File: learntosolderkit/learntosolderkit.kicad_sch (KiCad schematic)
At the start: 11 parts, among them J1 Barrel_Jack, SW1 SW_Push, SW2 SW_Push, SW3 SW_Push, U1 NE555P

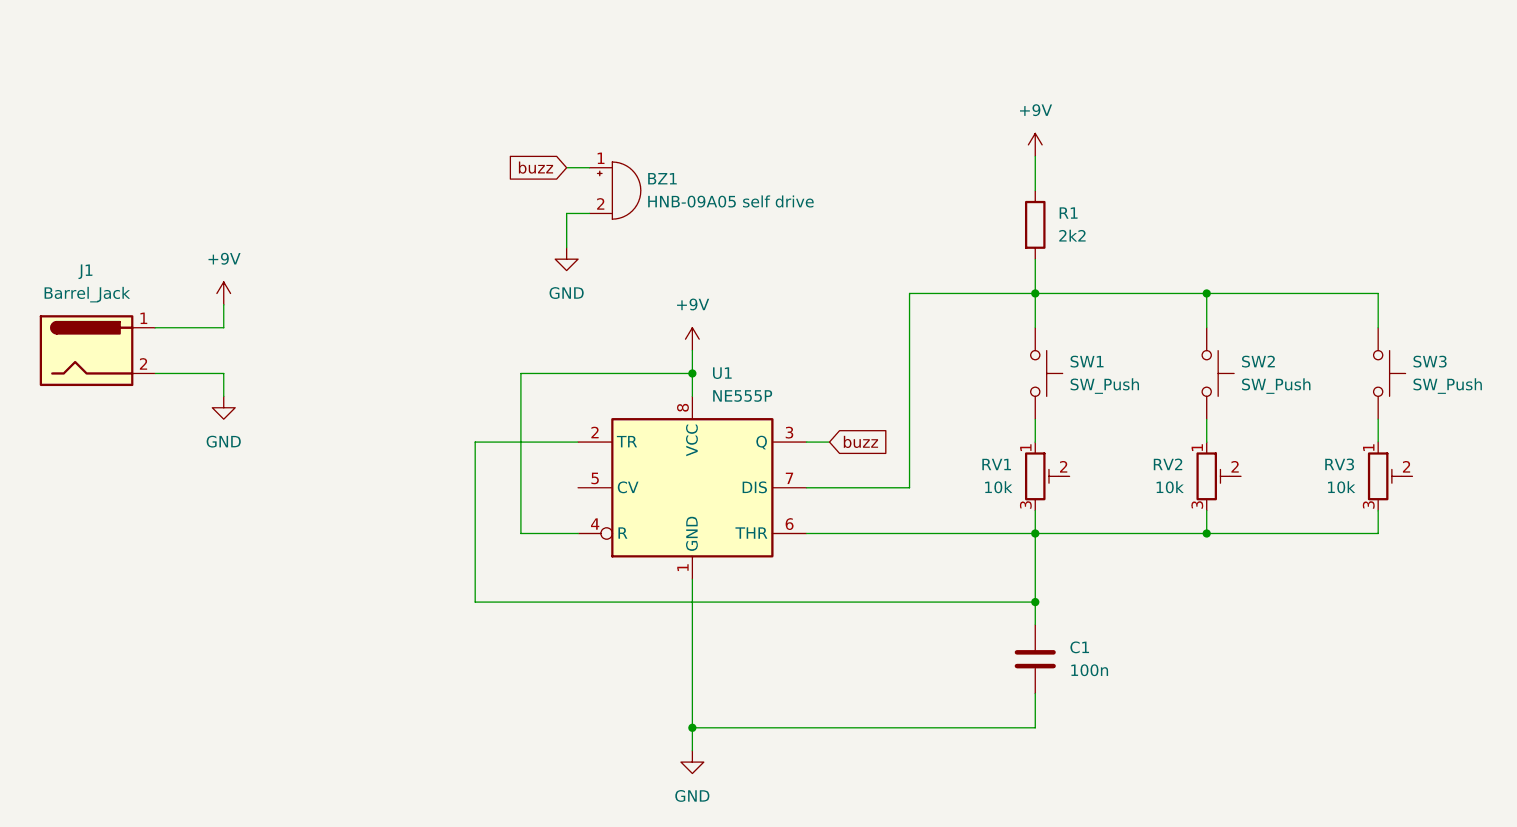
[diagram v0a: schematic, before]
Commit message: Finish up
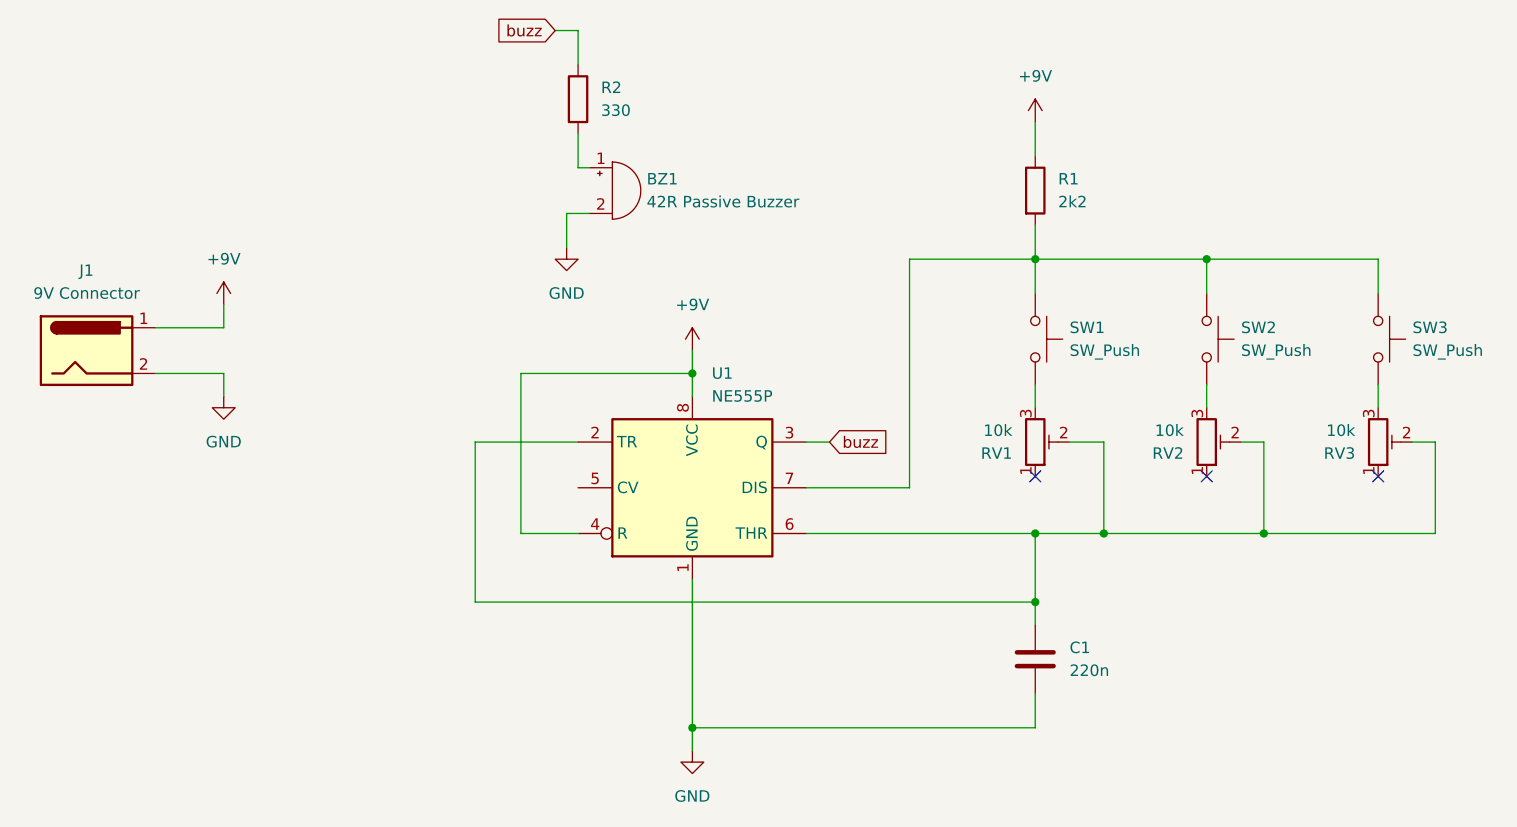
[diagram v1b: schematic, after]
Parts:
- added R2: 330, Resistor_THT:R_Axial_DIN0207_L6.3mm_D2.5mm_P10.16mm_Horizontal, symbol Device:R
- BZ1: value HNB-09A05 self drive -> 42R Passive Buzzer
- C1: value 100n -> 220n
- J1: value Barrel_Jack -> 9V Connector; footprint aaaa_custom:9V Battery Connection2THT -> 1_my_custom_library:9v_dc_batt_2_pin
- RV1, RV2, RV3: footprint Potentiometer_THT:Potentiometer_Runtron_RM-065_Vertical -> 1_my_custom_library:3386P_Trimmer
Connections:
- net buzz: now also R2.1; no longer BZ1.1 (+)
- net at RV3.1: no longer SW3.2
- net at RV3.2: now also C1.1, RV1.2, RV2.2, U1.2 (TR), U1.6 (THR)
- net at RV1.1: no longer SW1.2
- net at SW2.2: now also RV2.3; no longer RV2.1
- new net: RV3.3, SW3.2
- new net: RV1.3, SW1.2
- new net: BZ1.1 (+), R2.2
- no-connect marks 0 -> 3
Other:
- moved on the sheet: R1, RV1, RV2, RV3, SW1, SW2, SW3
